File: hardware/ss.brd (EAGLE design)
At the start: 65 x 62 mm, 85 parts, among them IC1 DS3231, Q1 BSS138, Q2 si2305cd, Q4 si2305cd, Q5 8MHz, Q6 si2305cd, T1 BC846, U1 SPX5205 3v3, U17 AVR_SPI_PRG_6PTH, U2 CN3083, U3 SPX5205 3v3, U5 ATMEGA328, U6 microSD Socket, X1 USBSMD

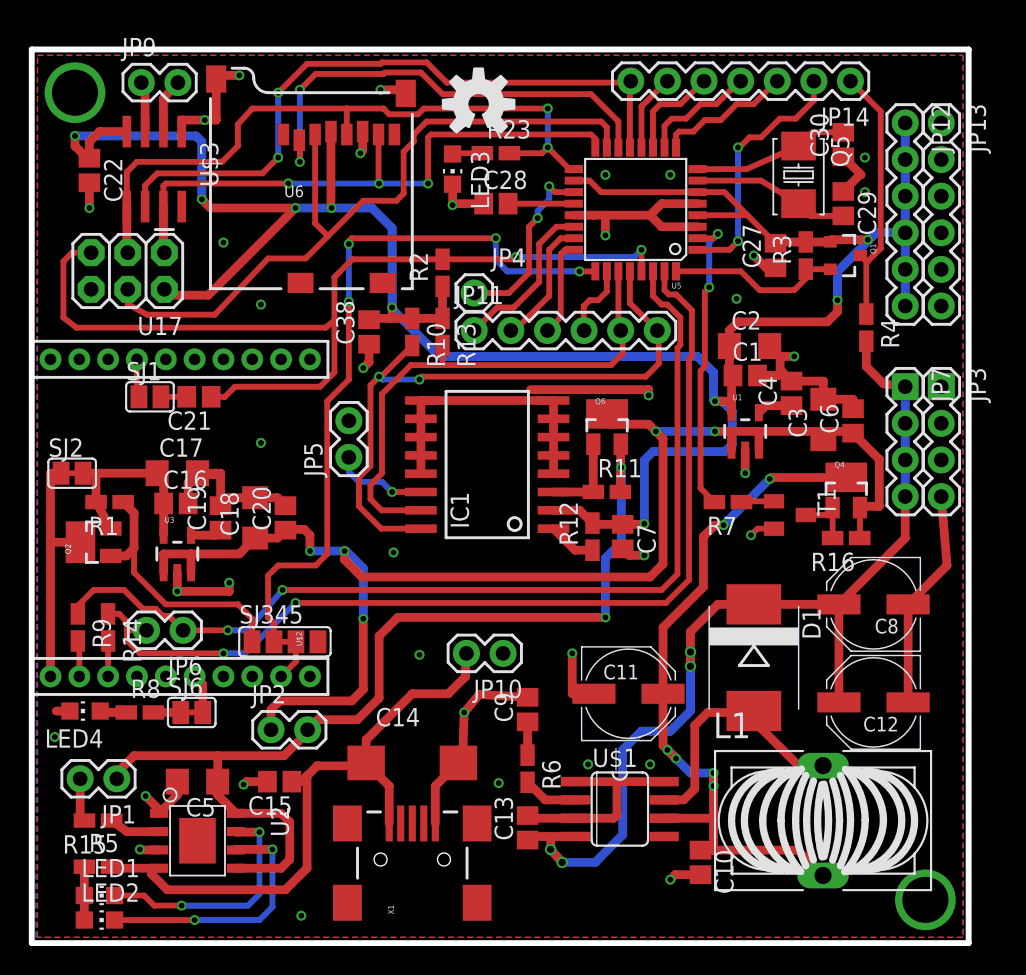
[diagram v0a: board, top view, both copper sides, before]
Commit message: latest
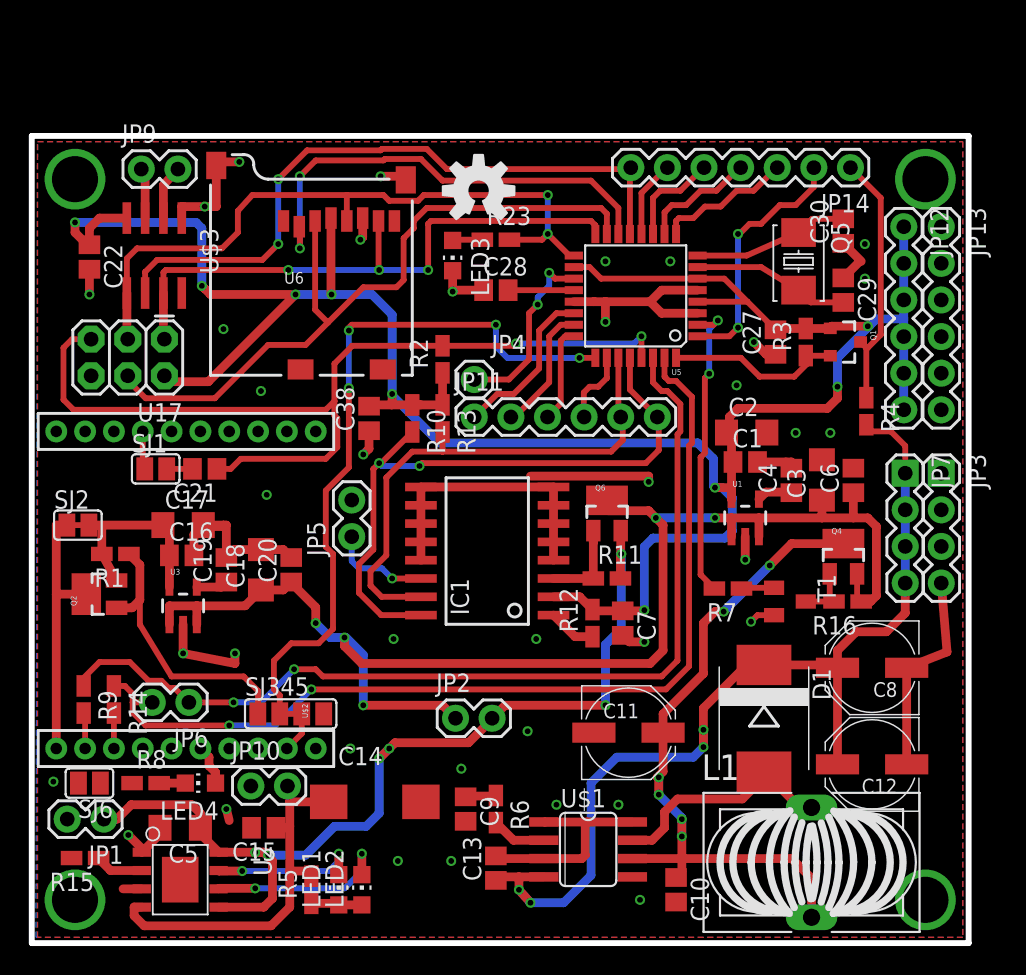
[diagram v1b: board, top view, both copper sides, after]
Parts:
- removed X1: USBSMD, SparkFun-Connectors:USB-MINIB
- moved JP10 19.8 mm to (15.2, 10.9), turned to 0 degrees
- moved LED2 18.3 mm to (22.9, 3.70), turned to 0 degrees
- moved LED1 16.6 mm to (21.3, 3.70), turned to 0 degrees
- moved R5 14.9 mm to (19.4, 3.70), turned to 90 degrees
- moved JP2 12.8 mm to (29.4, 15.6)
- moved LED4 9.43 mm to (11.7, 11.1)
- moved SJ6 8.63 mm to (4.00, 11.1), turned to 180 degrees
- moved C9 8.13 mm to (30.1, 9.30), turned to 270 degrees
- moved JP12 7.20 mm to (60.5, 49.7)
- moved JP13 7.20 mm to (63.1, 49.7)
- moved C4 6.04 mm to (52.7, 32.1)
- moved C2 6.00 mm to (49.6, 35.4)
- moved IC1 6.00 mm to (31.6, 27.2)
- moved C1 6.00 mm to (49.5, 33.4)
- moved C22 6.00 mm to (4.00, 47.6)
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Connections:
- removed net N$23: LED4.A, R8.1
- new net N$6: LED4.C, R8.2
- net GND: now also R8.1, SJ6.1, SJ6.2; no longer LED4.C, X1.GND
- net N$12: no longer X1.VBUS
- net N$7: now also LED4.A; no longer R8.2, SJ6.1, SJ6.2
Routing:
- net GND: track 163.3 -> 128.2 mm, vias 39 -> 42
- net N$12: track 44.5 -> 26.6 mm
- net N$15: track 16.6 -> 10.6 mm
- net N$16: track 17.9 -> 13.1 mm
- net N$7: track 6.19 -> 2.83 mm
- net VIN: track 99.3 -> 96.6 mm
- net BOOST_IN: track 52.2 -> 50.2 mm
- net V+: track 70.7 -> 68.8 mm, vias 2 -> 6
- net N$23: track 1.85 -> 0.00 mm
- net N$6: track 0.00 -> 1.81 mm
- net N$3: track 18.1 -> 16.3 mm
- net +3V3_XBEE: track 32.3 -> 33.7 mm
- net RST: track 64.7 -> 63.5 mm
- net XBEE_HIB: track 55.3 -> 54.1 mm
- net XBEE_PWR_SW_M: track 18.2 -> 19.3 mm
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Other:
- board size 65 x 62 mm -> 65 x 56 mm
- board text added: "+3v7"
- board text added: "ch"
- board text added: "fl"
- board text added: "power"
- board text added: "switch"
- board text removed: "+3.7v Lipo"
- board text removed: "charging"
- board text removed: "full"
- board text removed: "pw sw"

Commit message: hopefully flawless
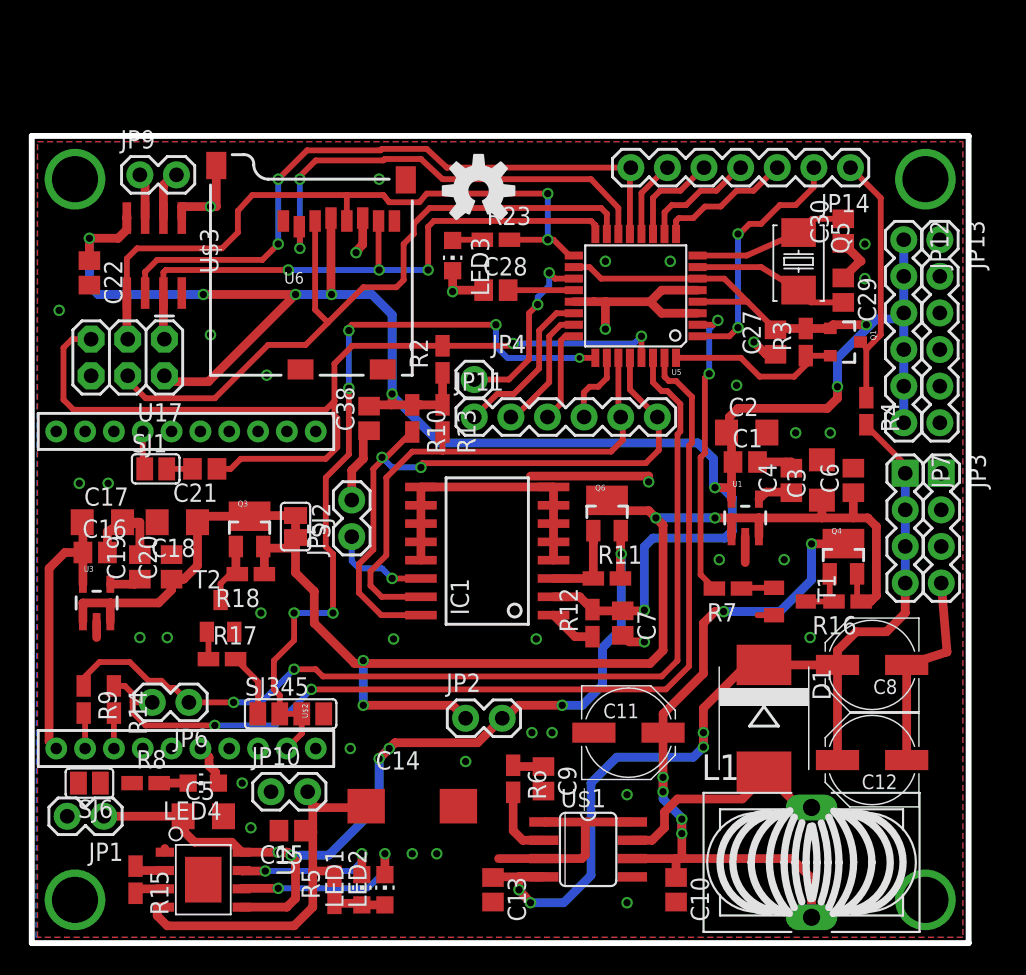
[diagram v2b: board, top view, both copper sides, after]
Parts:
- removed Q2: si2305cd, Simplex-DiscreteSemi:SOT23-3_POWER
- removed R1: 100k, rcl:R0805W
- added Q3: si2305cd, Simplex-DiscreteSemi:SOT23-3_POWER
- added R17: 1M, rcl:R0805W
- added R18: 100k, rcl:R0805W
- added T2: BC846, transistor:SOT23
- R7: value 100k -> 1M
- moved SJ2 15.1 mm to (18.3, 28.9), turned to 270 degrees
- moved C20 8.30 mm to (9.70, 26.1)
- moved C18 6.67 mm to (10.1, 29.2), turned to 180 degrees
- moved C16 6.00 mm to (4.40, 27.1)
- moved C19 6.00 mm to (7.50, 26.1)
- moved U3 6.00 mm to (4.50, 23.6)
- moved C9 5.79 mm to (35.5, 11.4)
- moved C17 5.60 mm to (4.90, 29.2)
- moved R15 3.81 mm to (7.20, 4.40), turned to 270 degrees
- moved C14 2.62 mm to (26.4, 9.50)
- moved R6 2.42 mm to (33.4, 11.4)
- moved C15 1.91 mm to (18.0, 7.80)
- moved C5 1.79 mm to (11.9, 8.80), turned to 0 degrees
- moved LED2 1.60 mm to (24.5, 3.70)
- moved R5 1.60 mm to (21.0, 3.70)
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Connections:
- new net N$18: R17.1, T2.1
- new net N$20: Q3.1, R18.2, T2.3
- net +3V3_XBEE: no longer Q2.2, Q2.3, R1.2, SJ2.1, SJ2.2
- net GND: now also T2.2
- net VIN: now also Q3.2, Q3.3, R18.1, SJ2.1, SJ2.2
- net XBEE_PWR_SW_M: now also R17.2; no longer Q2.1, R1.1
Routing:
- net VIN: track 96.6 -> 114.7 mm, vias 5 -> 4
- net XBEE_PWR_SW_M: track 19.3 -> 4.45 mm
- net GND: track 128.2 -> 114.2 mm
- net +3V3_XBEE: track 33.7 -> 19.8 mm
- net N$20: track 0.00 -> 4.53 mm
- net +3V3: track 176.4 -> 173.7 mm
- net V+: track 68.8 -> 66.5 mm
- net N$18: track 0.00 -> 1.95 mm
- net N$11: track 3.83 -> 5.06 mm
- net N$9: track 3.43 -> 2.34 mm
- net +5V: track 70.4 -> 70.9 mm
- net XBEE_HIB: track 54.1 -> 54.6 mm, vias 4 -> 6
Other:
- board text added: "+3v"
- board text added: "ok"
- board text added: "power sw"
- board text added: "sck"
- board text added: "t+"
- board text added: "t-"
- board text removed: "+3V Li"
- board text removed: "fl"
- board text removed: "power"
- board text removed: "switch"
